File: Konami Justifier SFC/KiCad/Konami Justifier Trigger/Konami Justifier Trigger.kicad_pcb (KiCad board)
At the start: 4 copper layers, 15.2 x 16.2 mm, 4 parts, among them SW1 SW_Push_Open

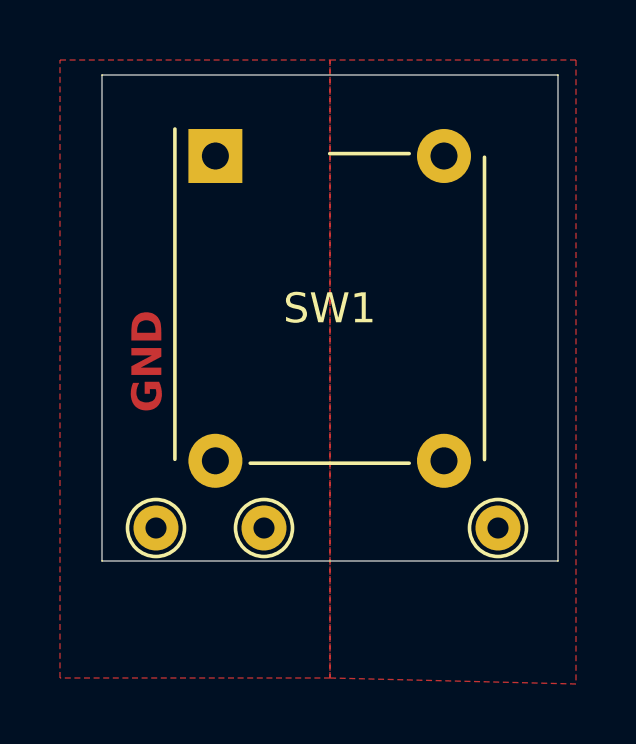
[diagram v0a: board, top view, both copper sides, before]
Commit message: Add files via upload
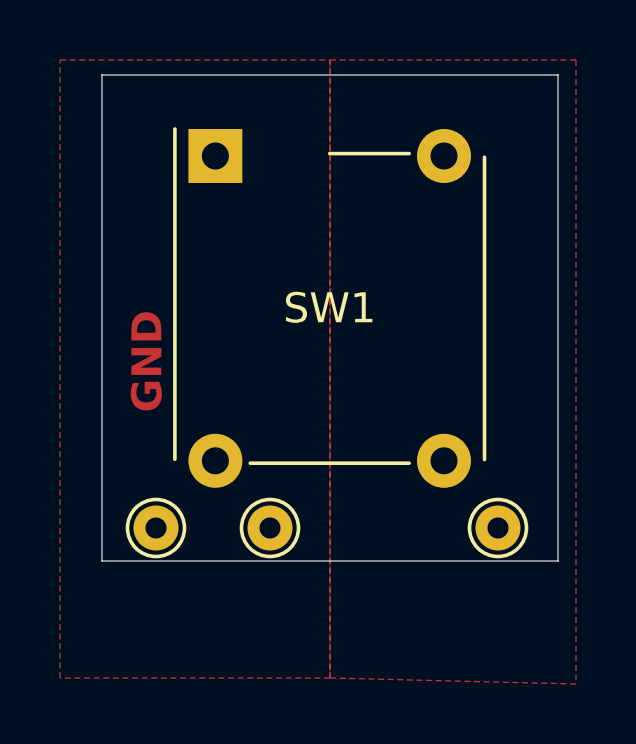
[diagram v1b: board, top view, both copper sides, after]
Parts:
- moved TP2 0.20 mm to (118.0, 106.6)
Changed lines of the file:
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@@
 	(footprint "TestPoint:TestPoint_THTPad_D1.5mm_Drill0.7mm"
 		(layer "F.Cu")
-		(at 117.8 106.6)
+		(at 118 106.6)
 		(descr "THT pad as test Point, diameter 1.5mm, hole diameter 0.7mm")
 		(tags "test point THT pad")
